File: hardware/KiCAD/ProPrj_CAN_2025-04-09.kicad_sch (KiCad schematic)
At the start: 26 parts, among them J1 KF2510-4, J2 Programm, J3 BOOT, J4 RESET, U1 LM2575-5.0BT, U2 AMS1117-3.3, U3 TJA1050DRG, U4 ESP-12F

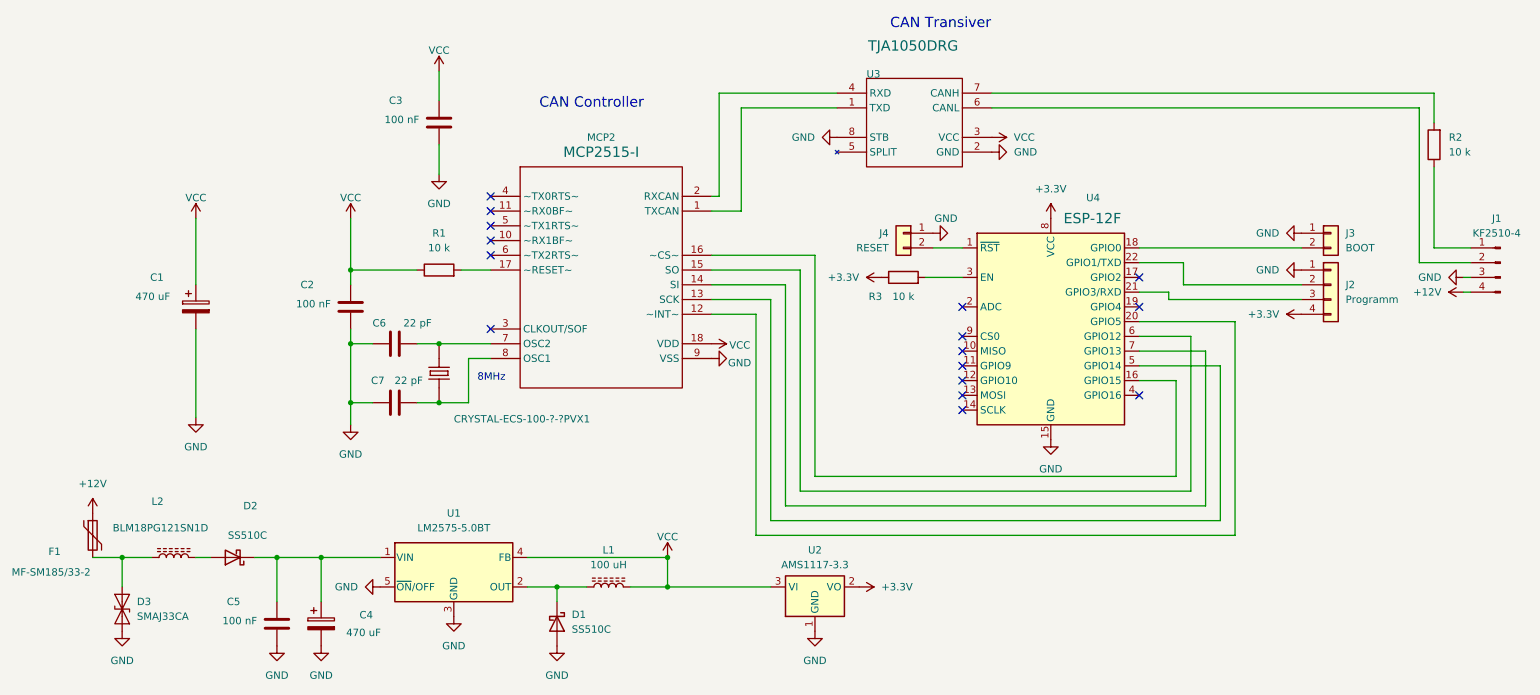
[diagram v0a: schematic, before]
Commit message: reorder
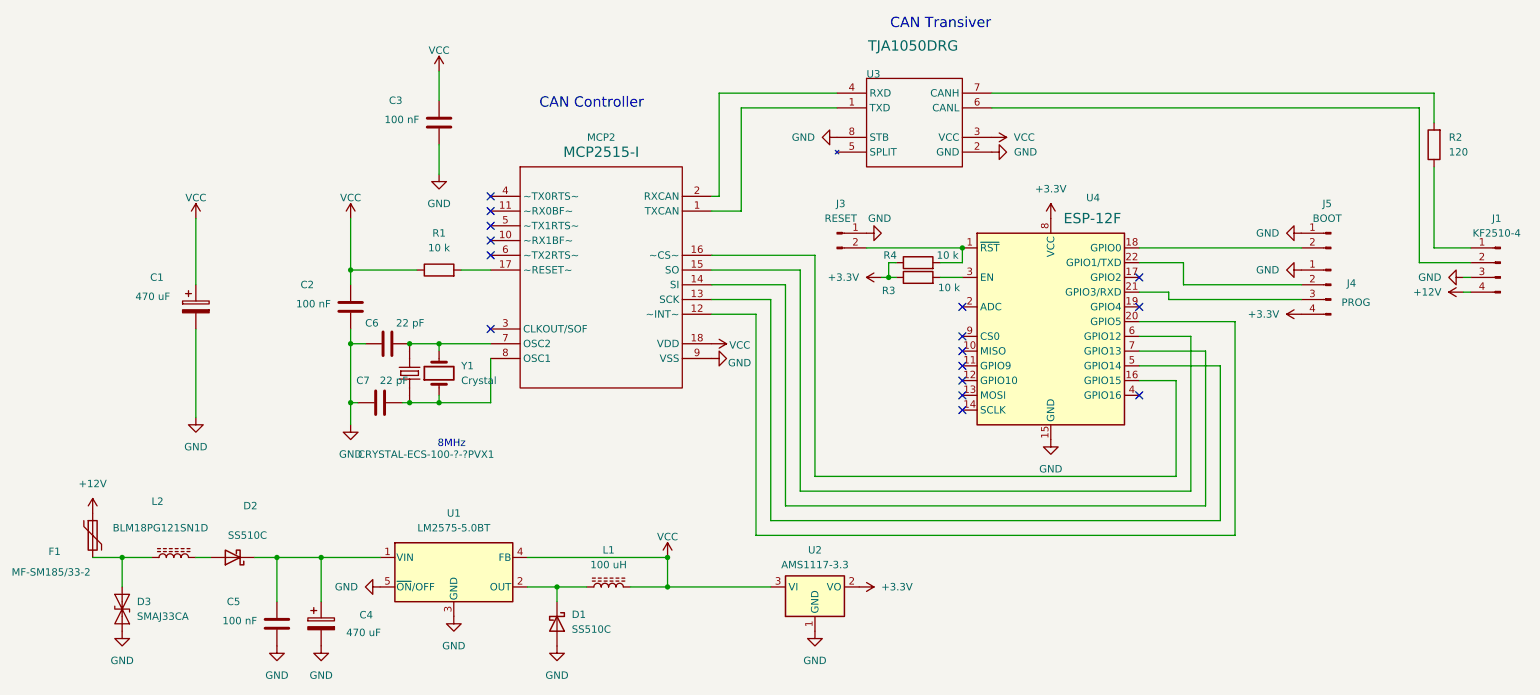
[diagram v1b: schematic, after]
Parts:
- removed J2: Programm, symbol Connector_Generic:Conn_01x04
- removed J3: BOOT, symbol Connector_Generic:Conn_01x02
- removed J4: RESET, symbol Connector_Generic:Conn_01x02
- added J3: RESET, Connector_PinSocket_2.54mm:PinSocket_1x02_P2.54mm_Vertical, symbol Connector:Conn_01x02_Pin
- added J4: PROG, Connector_PinHeader_2.54mm:PinHeader_1x04_P2.54mm_Vertical, symbol Connector:Conn_01x04_Pin
- added J5: BOOT, Connector_PinSocket_2.54mm:PinSocket_1x02_P2.54mm_Vertical, symbol Connector:Conn_01x02_Pin
- added R4: 10 k, Resistor_SMD:R_0603_1608Metric_Pad0.98x0.95mm_HandSolder, symbol Device:R
- added Y1: Crystal, Crystal:Crystal_SMD_HC49-SD_HandSoldering, symbol Device:Crystal
- F1: footprint (none) -> Inductor_SMD:L_0603_1608Metric_Pad1.05x0.95mm_HandSolder
- J1: footprint (none) -> Connector_Molex:Molex_KK-254_AE-6410-04A_1x04_P2.54mm_Vertical
- L1: footprint Inductor_SMD:L_12x12mm_H8mm -> Inductor_SMD:L_SXN_SMDRI127
- L2: footprint Inductor_SMD:L_0201_0603Metric_Pad0.64x0.40mm_HandSolder -> Inductor_SMD:L_0603_1608Metric_Pad1.05x0.95mm_HandSolder
- R2: value 10 k -> 120
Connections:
- net +3.3V: now also J4.4 (Pin_4), R4.1
- net GND: now also J3.1 (Pin_1), J4.1 (Pin_1), J5.1 (Pin_1)
- net at C6.2, CRYSTAL-ECS-100-?-?PVX1.2, MCP2.7 (OSC2): now also Y1.2
- net at U4.18 (GPIO0): now also J5.2 (Pin_2)
- net at C7.2, CRYSTAL-ECS-100-?-?PVX1.1, MCP2.8 (OSC1): now also Y1.1
- net at U4.1 (~{RST}): now also J3.2 (Pin_2), R4.2
- net at U4.21 (GPIO3/RXD): now also J4.3 (Pin_3)
- net at U4.22 (GPIO1/TXD): now also J4.2 (Pin_2)
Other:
- moved on the sheet: C6, C7, CRYSTAL-ECS-100-?-?PVX1, R3
